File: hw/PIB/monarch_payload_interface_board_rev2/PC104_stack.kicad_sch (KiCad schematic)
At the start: 35 parts, among them U1 Payload, U10 AD7124-8BCPZ-RL, U11 WSK06121L000FEA, U12 WSK06121L000FEA, U13 WSK06121L000FEA

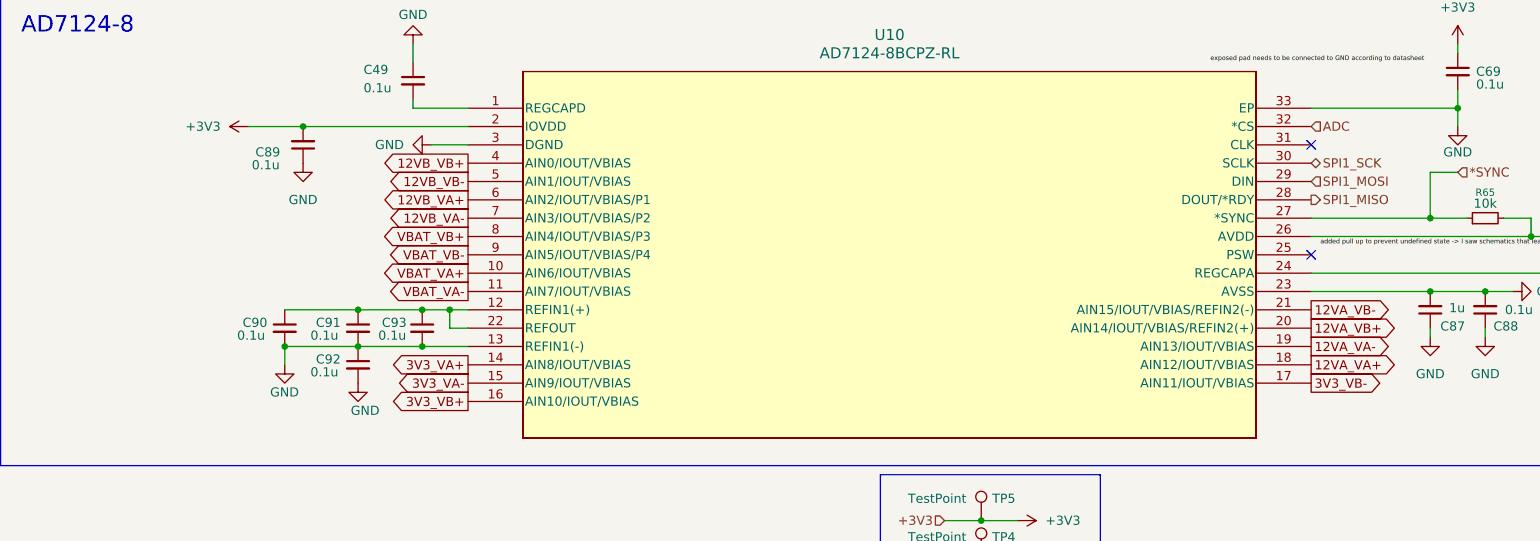
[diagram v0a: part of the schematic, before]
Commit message: Great progress almost done
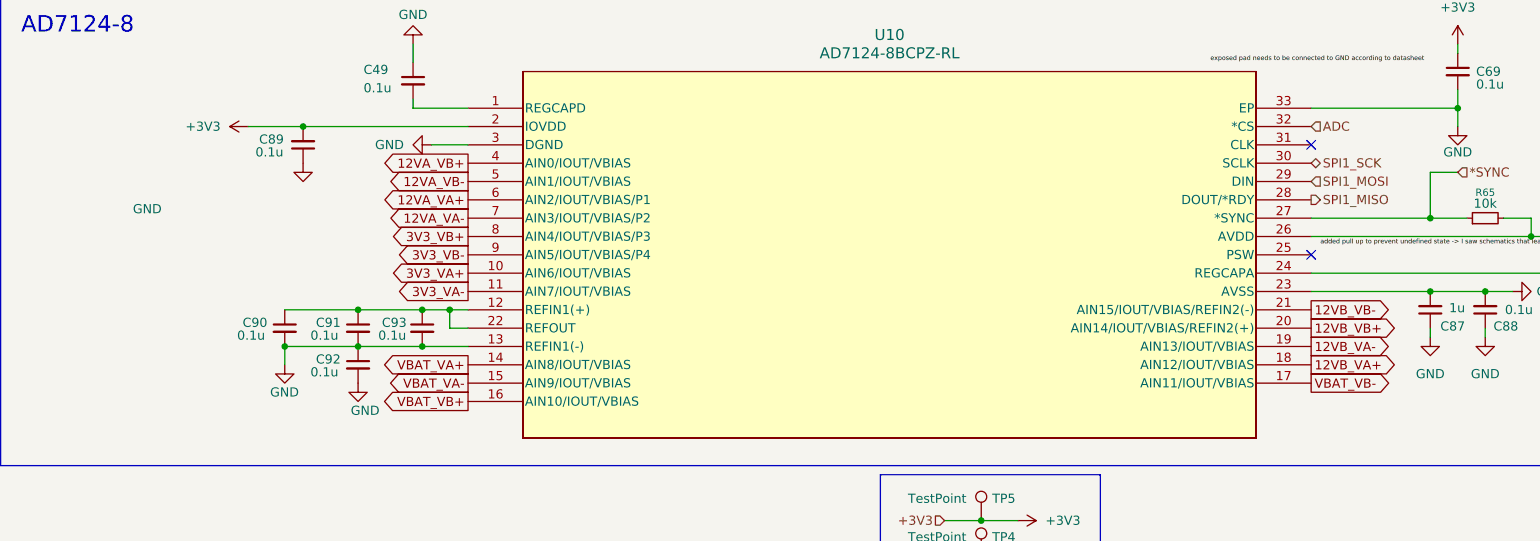
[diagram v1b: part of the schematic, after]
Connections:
- net 12VA_VA+: now also U10.6 (AIN2/IOUT/VBIAS/P1); no longer U10.18 (AIN12/IOUT/VBIAS)
- net 12VA_VB+: now also U10.4 (AIN0/IOUT/VBIAS); no longer U10.20 (AIN14/IOUT/VBIAS/REFIN2(+))
- net 12VB_VA+: now also U10.18 (AIN12/IOUT/VBIAS); no longer U10.6 (AIN2/IOUT/VBIAS/P1)
- net 12VB_VA-: now also U10.19 (AIN13/IOUT/VBIAS); no longer U10.7 (AIN3/IOUT/VBIAS/P2)
- net 12VB_VB+: now also U10.20 (AIN14/IOUT/VBIAS/REFIN2(+)); no longer U10.4 (AIN0/IOUT/VBIAS)
- net 12VB_VB-: now also U10.21 (AIN15/IOUT/VBIAS/REFIN2(-)); no longer U10.5 (AIN1/IOUT/VBIAS)
- net 3V3_VA+: now also U10.10 (AIN6/IOUT/VBIAS); no longer U10.14 (AIN8/IOUT/VBIAS)
- net 3V3_VB+: now also U10.8 (AIN4/IOUT/VBIAS/P3); no longer U10.16 (AIN10/IOUT/VBIAS)
- net GND: now also U10.5 (AIN1/IOUT/VBIAS), U10.7 (AIN3/IOUT/VBIAS/P2); no longer U10.19 (AIN13/IOUT/VBIAS), U10.21 (AIN15/IOUT/VBIAS/REFIN2(-))
- net VBAT_VA+: now also U10.14 (AIN8/IOUT/VBIAS); no longer U10.10 (AIN6/IOUT/VBIAS)
- net VBAT_VB+: now also U10.16 (AIN10/IOUT/VBIAS); no longer U10.8 (AIN4/IOUT/VBIAS/P3)
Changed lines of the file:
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@@
 	)
 	(junction
-		(at 220.98 138.43)
-		(diameter 0)
-		(color 0 0 0 0)
-	)
-	(junction
 		(at 62.23 146.05)
 		(diameter 0)
@@
 	)
 	(junction
+		(at 220.98 138.43)
+		(diameter 0)
+		(color 0 0 0 0)
+	)
+	(junction
 		(at 214.63 30.48)
 		(diameter 0)
@@
 	(global_label "12VA_VA-"
 		(shape output)
-		(at 204.47 146.05 0)
+		(at 87.63 128.27 180)
 		(fields_autoplaced yes)
 		(effects
@@
 				(size 1.27 1.27)
 			)
-			(justify left)
+			(justify right)
 		)
 		(property "Intersheetrefs" "${INTERSHEET_REFS}"
-			(at 216.1144 146.05 0)
+			(at 75.9856 128.27 0)
 			(hide yes)
 			(show_name no)
@@
 					(size 1.27 1.27)
 				)
-				(justify left)
+				(justify right)
 			)
 		)
@@
 	(global_label "3V3_VA+"
 		(shape output)
-		(at 87.63 148.59 180)
+		(at 87.63 135.89 180)
 		(fields_autoplaced yes)
 		(effects
@@
 		)
 		(property "Intersheetrefs" "${INTERSHEET_REFS}"
-			(at 77.0742 148.59 0)
+			(at 77.0742 135.89 0)
 			(hide yes)
 			(show_name no)
@@
 	(global_label "VBAT_VB-"
 		(shape output)
-		(at 87.63 133.35 180)
+		(at 204.47 151.13 0)
 		(fields_autoplaced yes)
 		(effects
@@
 				(size 1.27 1.27)
 			)
-			(justify right)
+			(justify left)
 		)
 		(property "Intersheetrefs" "${INTERSHEET_REFS}"
-			(at 75.9856 133.35 0)
+			(at 216.1144 151.13 0)
 			(hide yes)
 			(show_name no)
@@
 					(size 1.27 1.27)
 				)
-				(justify right)
+				(justify left)
 			)
 		)
@@
 	(global_label "3V3_VB-"
 		(shape output)
-		(at 204.47 151.13 0)
+		(at 87.63 133.35 180)
 		(fields_autoplaced yes)
 		(effects
@@
 				(size 1.27 1.27)
 			)
-			(justify left)
+			(justify right)
 		)
 		(property "Intersheetrefs" "${INTERSHEET_REFS}"
-			(at 215.2072 151.13 0)
+			(at 76.8928 133.35 0)
 			(hide yes)
 			(show_name no)
@@
 					(size 1.27 1.27)
 				)
-				(justify left)
+				(justify right)
 			)
 		)
@@
 	(global_label "12VA_VB+"
 		(shape output)
-		(at 204.47 143.51 0)
+		(at 87.63 120.65 180)
 		(fields_autoplaced yes)
 		(effects
@@
 				(size 1.27 1.27)
 			)
-			(justify left)
+			(justify right)
 		)
 		(property "Intersheetrefs" "${INTERSHEET_REFS}"
-			(at 216.2958 143.51 0)
+			(at 75.8042 120.65 0)
 			(hide yes)
 			(show_name no)
@@
 					(size 1.27 1.27)
 				)
-				(justify left)
+				(justify right)
 			)
 		)
@@
 	(global_label "VBAT_VA-"
 		(shape output)
-		(at 87.63 138.43 180)
+		(at 87.63 151.13 180)
 		(fields_autoplaced yes)
 		(effects
@@
 		)
 		(property "Intersheetrefs" "${INTERSHEET_REFS}"
-			(at 76.167 138.43 0)
+			(at 76.167 151.13 0)
 			(hide yes)
 			(show_name no)
@@
 	(global_label "3V3_VB+"
 		(shape output)
-		(at 87.63 153.67 180)
+		(at 87.63 130.81 180)
 		(fields_autoplaced yes)
 		(effects
@@
 		)
 		(property "Intersheetrefs" "${INTERSHEET_REFS}"
-			(at 76.8928 153.67 0)
+			(at 76.8928 130.81 0)
 			(hide yes)
 			(show_name no)
@@
 	(global_label "VBAT_VB+"
 		(shape output)
-		(at 87.63 130.81 180)
+		(at 87.63 153.67 180)
 		(fields_autoplaced yes)
 		(effects
@@
 		)
 		(property "Intersheetrefs" "${INTERSHEET_REFS}"
-			(at 75.9856 130.81 0)
+			(at 75.9856 153.67 0)
 			(hide yes)
 			(show_name no)
@@
 	(global_label "VBAT_VA+"
 		(shape output)
-		(at 87.63 135.89 180)
+		(at 87.63 148.59 180)
 		(fields_autoplaced yes)
 		(effects
@@
 		)
 		(property "Intersheetrefs" "${INTERSHEET_REFS}"
-			(at 76.167 135.89 0)
+			(at 76.167 148.59 0)
 			(hide yes)
 			(show_name no)
@@
 	(global_label "12VB_VB+"
 		(shape output)
-		(at 87.63 120.65 180)
+		(at 204.47 143.51 0)
 		(fields_autoplaced yes)
 		(effects
@@
 				(size 1.27 1.27)
 			)
-			(justify right)
+			(justify left)
 		)
 		(property "Intersheetrefs" "${INTERSHEET_REFS}"
-			(at 75.6228 120.65 0)
+			(at 216.4772 143.51 0)
 			(hide yes)
 			(show_name no)
@@
 					(size 1.27 1.27)
 				)
-				(justify right)
+				(justify left)
 			)
 		)
@@
 	(global_label "3V3_VA-"
 		(shape output)
-		(at 87.63 151.13 180)
+		(at 87.63 138.43 180)
 		(fields_autoplaced yes)
 		(effects
@@
 		)
 		(property "Intersheetrefs" "${INTERSHEET_REFS}"
-			(at 77.0742 151.13 0)
+			(at 77.0742 138.43 0)
 			(hide yes)
 			(show_name no)
@@
 	(global_label "12VB_VB-"
 		(shape output)
-		(at 87.63 123.19 180)
+		(at 204.47 140.97 0)
 		(fields_autoplaced yes)
 		(effects
@@
 				(size 1.27 1.27)
 			)
-			(justify right)
+			(justify left)
 		)
 		(property "Intersheetrefs" "${INTERSHEET_REFS}"
-			(at 75.6228 123.19 0)
+			(at 216.4772 140.97 0)
 			(hide yes)
 			(show_name no)
@@
 					(size 1.27 1.27)
 				)
-				(justify right)
+				(justify left)
 			)
 		)
@@
 	(global_label "12VB_VA-"
 		(shape output)
-		(at 87.63 128.27 180)
+		(at 204.47 146.05 0)
 		(fields_autoplaced yes)
 		(effects
@@
 				(size 1.27 1.27)
 			)
-			(justify right)
+			(justify left)
 		)
 		(property "Intersheetrefs" "${INTERSHEET_REFS}"
-			(at 75.8042 128.27 0)
+			(at 216.2958 146.05 0)
 			(hide yes)
 			(show_name no)
@@
 					(size 1.27 1.27)
 				)
-				(justify right)
+				(justify left)
 			)
 		)
@@
 	(global_label "12VA_VA+"
 		(shape output)
-		(at 204.47 148.59 0)
+		(at 87.63 125.73 180)
 		(fields_autoplaced yes)
 		(effects
@@
 				(size 1.27 1.27)
 			)
-			(justify left)
+			(justify right)
 		)
 		(property "Intersheetrefs" "${INTERSHEET_REFS}"
-			(at 216.1144 148.59 0)
+			(at 75.9856 125.73 0)
 			(hide yes)
 			(show_name no)
@@
 					(size 1.27 1.27)
 				)
-				(justify left)
+				(justify right)
 			)
 		)
@@
 	(global_label "12VA_VB-"
 		(shape output)
-		(at 204.47 140.97 0)
+		(at 87.63 123.19 180)
 		(fields_autoplaced yes)
 		(effects
@@
 				(size 1.27 1.27)
 			)
-			(justify left)
+			(justify right)
 		)
 		(property "Intersheetrefs" "${INTERSHEET_REFS}"
-			(at 216.2958 140.97 0)
+			(at 75.8042 123.19 0)
 			(hide yes)
 			(show_name no)
@@
 					(size 1.27 1.27)
 				)
-				(justify left)
+				(justify right)
 			)
 		)
@@
 	(global_label "12VB_VA+"
 		(shape output)
-		(at 87.63 125.73 180)
+		(at 204.47 148.59 0)
 		(fields_autoplaced yes)
 		(effects
@@
 				(size 1.27 1.27)
 			)
-			(justify right)
+			(justify left)
 		)
 		(property "Intersheetrefs" "${INTERSHEET_REFS}"
-			(at 75.8042 125.73 0)
+			(at 216.2958 148.59 0)
 			(hide yes)
 			(show_name no)
@@
 					(size 1.27 1.27)
 				)
-				(justify right)
+				(justify left)
 			)
 		)
@@
 		(dnp no)
 		(property "Reference" "C89"
-			(at 58.166 119.126 0)
+			(at 58.674 117.348 0)
 			(show_name no)
 			(do_not_autoplace no)
@@
 		)
 		(property "Value" "0.1u"
-			(at 57.658 120.904 0)
+			(at 58.166 119.126 0)
 			(show_name no)
 			(do_not_autoplace no)
@@
 		(in_pos_files yes)
 		(dnp no)
-		(fields_autoplaced yes)
 		(property "Reference" "#PWR0259"
 			(at 64.77 127 0)
@@
 		)
 		(property "Value" "GND"
-			(at 64.77 125.73 0)
+			(at 43.18 127 0)
 			(show_name no)
 			(do_not_autoplace no)
